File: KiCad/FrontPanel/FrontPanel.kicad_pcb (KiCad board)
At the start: 2 copper layers, 83 x 29 mm, 13 parts, among them J1 5V, J2 GND

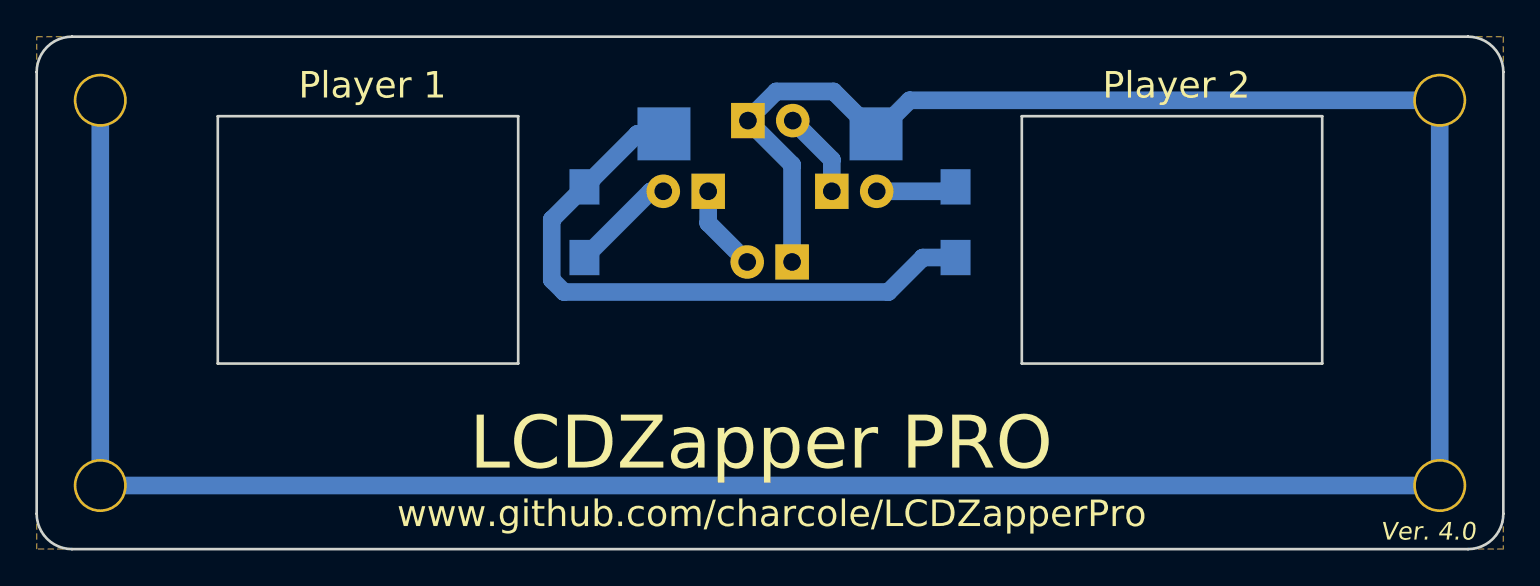
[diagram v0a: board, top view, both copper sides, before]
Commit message: Fixes based on print outs
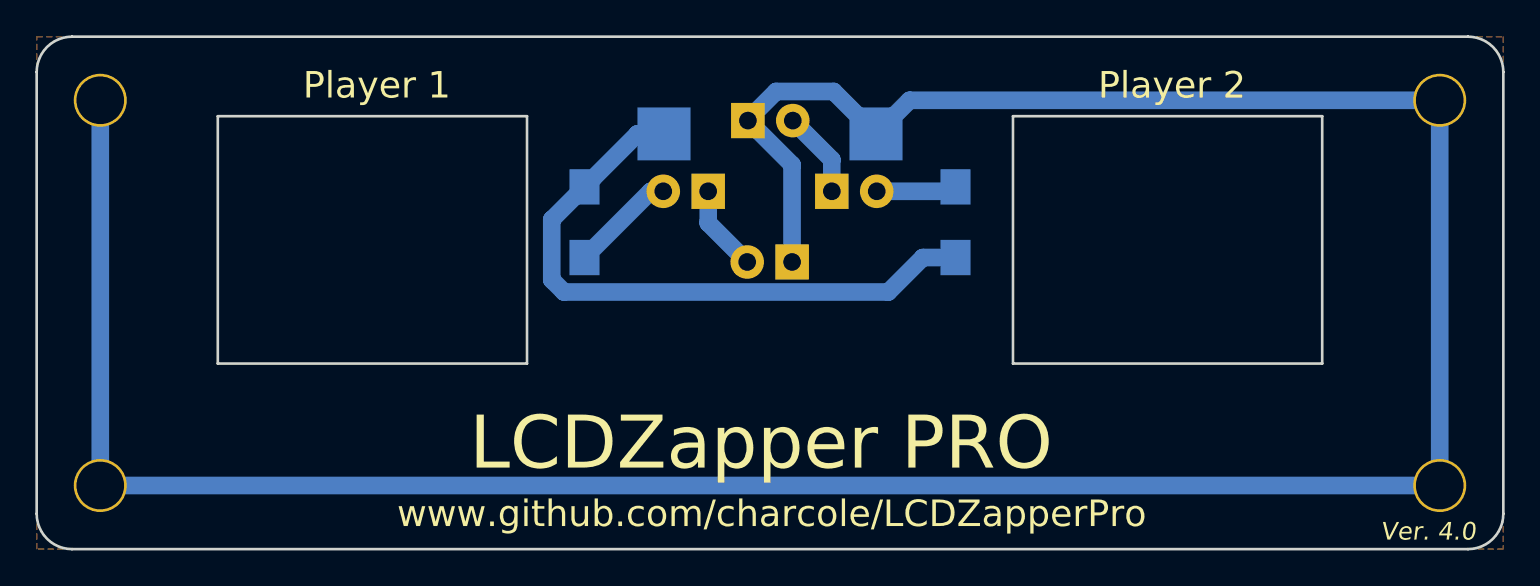
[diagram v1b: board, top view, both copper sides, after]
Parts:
- moved REF** 0.25 mm to (141.2, 88.0)
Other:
- outline, holes or cut-outs redrawn
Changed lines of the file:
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@@
     (mod_text_size 1 1)
     (mod_text_width 0.15)
-    (pad_size 3 3)
-    (pad_drill 2.7)
+    (pad_size 20 1.8)
+    (pad_drill 20)
     (pad_to_mask_clearance 0.2)
     (aux_axis_origin 0 0)
@@
   )
   (module Mounting_Holes:MountingHole_2.7mm_M2.5 (layer F.Cu)
-    (at 141.5 88)
+    (at 141.25 88)
     (descr "Mounting Hole 2.7mm, no annular, M2.5")
     (tags "mounting hole 2.7mm no annular m2.5")
@@
     (fp_circle (center 0 0) (end 2.7 0) (layer Cmts.User) (width 0.15))
     (fp_circle (center 0 0) (end 2.95 0) (layer F.CrtYd) (width 0.05))
-    (pad "" np_thru_hole oval (at 0 0) (size 18 1.8) (drill oval 18 1.8) (layers *.Cu *.Mask))
+    (pad "" np_thru_hole oval (at 0 0) (size 20 1.8) (drill oval 20 1.8) (layers *.Cu *.Mask))
   )
   (module LEDs:LED-5MM (layer B.Cu)
@@
     (effects (font (size 1.5 1.5) (thickness 0.3)) (justify mirror))
   )
-  (gr_line (start 155.75 74.5) (end 155.75 88.5) (layer Edge.Cuts) (width 0.15))
+  (gr_line (start 155.25 74.5) (end 155.25 88.5) (layer Edge.Cuts) (width 0.15))
   (gr_line (start 172.75 88.5) (end 172.75 74.5) (layer Edge.Cuts) (width 0.15))
-  (gr_line (start 172.75 74.5) (end 155.75 74.5) (layer Edge.Cuts) (width 0.15))
-  (gr_line (start 172.75 88.5) (end 155.75 88.5) (layer Edge.Cuts) (width 0.15))
+  (gr_line (start 172.75 74.5) (end 155.25 74.5) (layer Edge.Cuts) (width 0.15))
+  (gr_line (start 172.75 88.5) (end 155.25 88.5) (layer Edge.Cuts) (width 0.15))
   (dimension 76.5 (width 0.3) (layer Eco2.User)
     (gr_text "76.500 mm" (at 141.482159 118.59496) (layer Eco2.User)
@@
     (arrow2b (pts (xy 100 107.5) (xy 101.126504 106.913579)))
   )
-  (gr_line (start 127.25 88.5) (end 110.25 88.5) (layer Edge.Cuts) (width 0.15))
+  (gr_line (start 127.75 88.5) (end 110.25 88.5) (layer Edge.Cuts) (width 0.15))
   (gr_line (start 110.25 74.5) (end 110.25 88.5) (layer Edge.Cuts) (width 0.15))
-  (gr_line (start 127.25 74.5) (end 110.25 74.5) (layer Edge.Cuts) (width 0.15))
-  (gr_line (start 127.25 88.5) (end 127.25 74.5) (layer Edge.Cuts) (width 0.15))
+  (gr_line (start 127.75 74.5) (end 110.25 74.5) (layer Edge.Cuts) (width 0.15))
+  (gr_line (start 127.75 88.5) (end 127.75 74.5) (layer Edge.Cuts) (width 0.15))
   (gr_text "LCDZapper PRO" (at 141 93) (layer F.SilkS)
     (effects (font (size 3 3) (thickness 0.75)))
   )
-  (gr_text "Player 2" (at 164.5 72.75) (layer F.SilkS)
+  (gr_text "Player 2" (at 164.25 72.75) (layer F.SilkS)
     (effects (font (size 1.5 1.5) (thickness 0.3)))
   )
-  (gr_text "Player 1" (at 119 72.75) (layer F.SilkS)
+  (gr_text "Player 1" (at 119.25 72.75) (layer F.SilkS)
     (effects (font (size 1.5 1.5) (thickness 0.3)))
   )
